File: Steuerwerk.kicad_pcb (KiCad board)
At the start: 2 copper layers, 100 x 160 mm, 332 parts, among them J1 Conn_01x04, J2 Conn_01x02, J3 Conn_01x03, J4 Conn_01x03, J5 Conn_01x02, J6 Conn_01x04, J7 Conn_01x02, J8 Conn_01x04, J9 Conn_01x02, Q1 Q_PNP_BCE, U1 74LS161, U2 74LS138, U3 74LS138, U4 74240, U5 74LS374, U6 74LS374, U7 74541, U8 74541

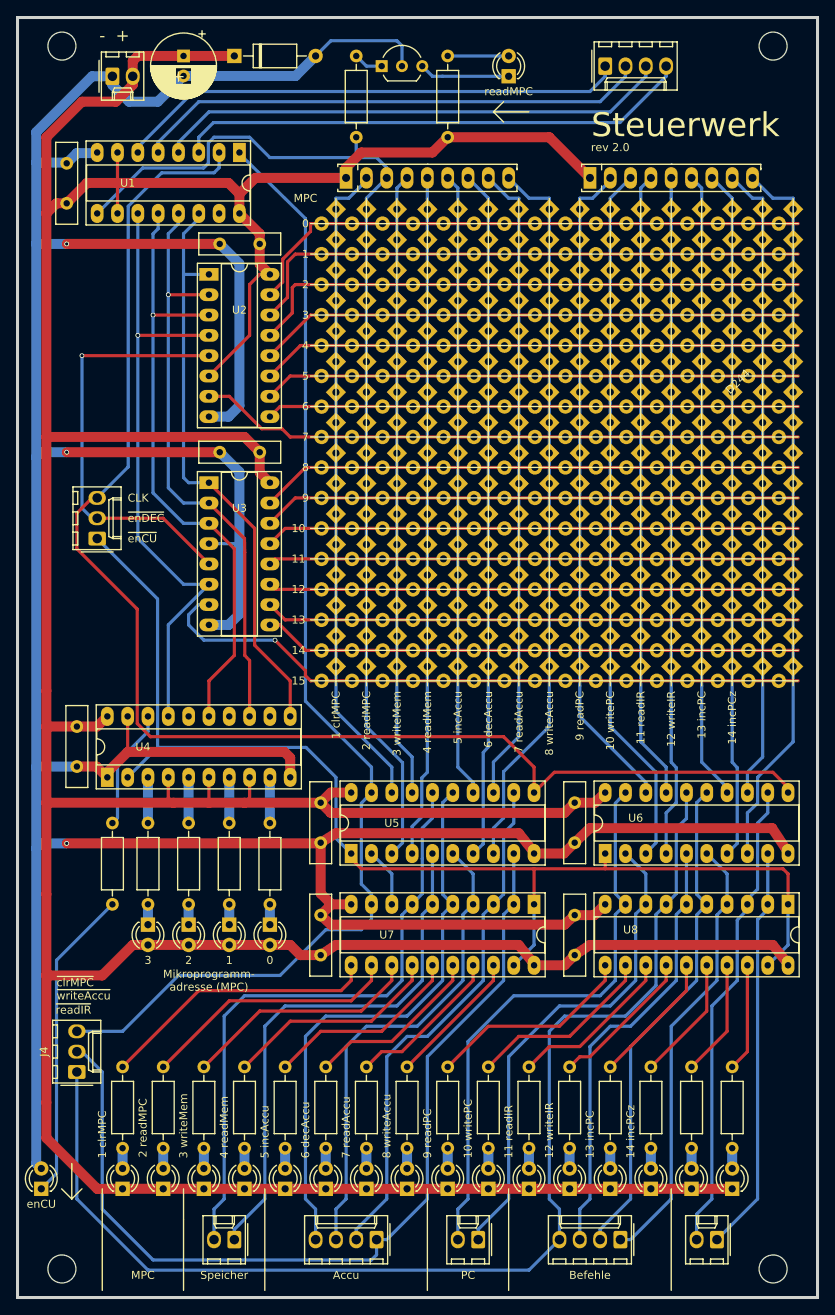
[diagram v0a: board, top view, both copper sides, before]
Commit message: Steuerwerk und Befehle bearbeitet
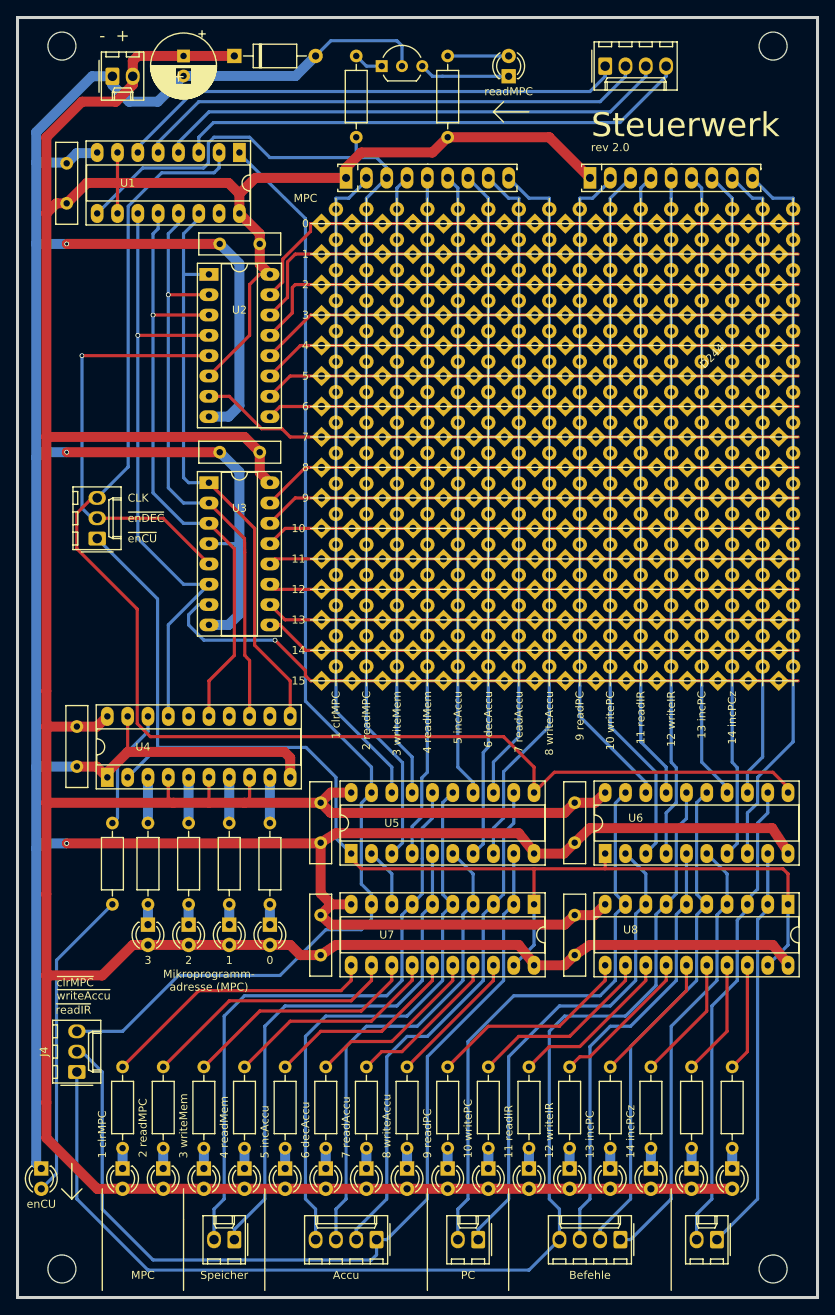
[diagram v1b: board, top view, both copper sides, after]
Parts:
- moved D12 2.55 mm to (87.1, 73.6), turned to 45 degrees
- moved D17 2.55 mm to (125.2, 77.4), turned to 45 degrees
- moved D41 2.55 mm to (121.4, 111.7), turned to 45 degrees
- moved D40 2.54 mm to (87.1, 111.7), turned to 45 degrees
- moved D47 2.54 mm to (44.5, 176.5), turned to 270 degrees
- moved D48 2.54 mm to (54.6, 176.5), turned to 270 degrees
- moved D49 2.54 mm to (59.7, 176.5), turned to 270 degrees
- moved D50 2.54 mm to (64.8, 176.5), turned to 270 degrees
- moved D51 2.54 mm to (69.9, 176.5), turned to 270 degrees
- moved D52 2.54 mm to (75.0, 176.5), turned to 270 degrees
- moved D53 2.54 mm to (80.0, 176.5), turned to 270 degrees
- moved D54 2.54 mm to (85.1, 176.5), turned to 270 degrees
- moved D55 2.54 mm to (90.2, 176.5), turned to 270 degrees
- moved D56 2.54 mm to (95.3, 176.5), turned to 270 degrees
- moved D57 2.54 mm to (100.4, 176.5), turned to 270 degrees
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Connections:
- D10 pad 1: Net-(D10-Pad1) -> /h6
- D10 pad 2: /h6 -> Net-(D10-Pad2)
- D100 pad 1: Net-(D100-Pad1) -> /h5
- D100 pad 2: /h5 -> Net-(D100-Pad2)
- D101 pad 1: Net-(D101-Pad1) -> /h5
- D101 pad 2: /h5 -> Net-(D101-Pad2)
- D102 pad 1: Net-(D102-Pad1) -> /h5
- D102 pad 2: /h5 -> Net-(D102-Pad2)
- D103 pad 1: Net-(D103-Pad1) -> /h5
- D103 pad 2: /h5 -> Net-(D103-Pad2)
- D104 pad 1: Net-(D104-Pad1) -> /h5
- D104 pad 2: /h5 -> Net-(D104-Pad2)
- D105 pad 1: Net-(D105-Pad1) -> /h5
- D105 pad 2: /h5 -> Net-(D105-Pad2)
- D106 pad 1: Net-(D100-Pad1) -> /h6
- D106 pad 2: /h6 -> Net-(D100-Pad2)
- D107 pad 1: Net-(D101-Pad1) -> /h6
- D107 pad 2: /h6 -> Net-(D101-Pad2)
- D108 pad 1: Net-(D108-Pad1) -> /h6
- D108 pad 2: /h6 -> Net-(D108-Pad2)
- D109 pad 1: Net-(D103-Pad1) -> /h6
- D109 pad 2: /h6 -> Net-(D103-Pad2)
- D11 pad 1: Net-(D11-Pad1) -> /h3
- D11 pad 2: /h3 -> Net-(D11-Pad2)
- D110 pad 1: Net-(D104-Pad1) -> /h6
- D110 pad 2: /h6 -> Net-(D104-Pad2)
- D111 pad 1: Net-(D10-Pad1) -> /h7
- D111 pad 2: /h7 -> Net-(D10-Pad2)
- D112 pad 1: Net-(D100-Pad1) -> /h7
- D112 pad 2: /h7 -> Net-(D100-Pad2)
- D113 pad 1: Net-(D101-Pad1) -> /h7
- D113 pad 2: /h7 -> Net-(D101-Pad2)
- D114 pad 1: Net-(D102-Pad1) -> /h7
- D114 pad 2: /h7 -> Net-(D102-Pad2)
- D115 pad 1: Net-(D108-Pad1) -> /h7
- D115 pad 2: /h7 -> Net-(D108-Pad2)
- D116 pad 1: Net-(D103-Pad1) -> /h7
- D116 pad 2: /h7 -> Net-(D103-Pad2)
- D117 pad 1: Net-(D104-Pad1) -> /h7
- D117 pad 2: /h7 -> Net-(D104-Pad2)
- D118 pad 1: Net-(D105-Pad1) -> /h7
- D118 pad 2: /h7 -> Net-(D105-Pad2)
- D119 pad 1: Net-(D10-Pad1) -> /h8
- D119 pad 2: /h8 -> Net-(D10-Pad2)
- D12 pad 1: Net-(D101-Pad1) -> /h4
- D12 pad 2: /h4 -> Net-(D101-Pad2)
- D120 pad 1: Net-(D100-Pad1) -> /h8
- D120 pad 2: /h8 -> Net-(D100-Pad2)
- D121 pad 1: Net-(D102-Pad1) -> /h8
- D121 pad 2: /h8 -> Net-(D102-Pad2)
- D122 pad 1: Net-(D108-Pad1) -> /h8
- D122 pad 2: /h8 -> Net-(D108-Pad2)
- D123 pad 1: Net-(D103-Pad1) -> /h8
- D123 pad 2: /h8 -> Net-(D103-Pad2)
- D124 pad 1: Net-(D105-Pad1) -> /h8
- D124 pad 2: /h8 -> Net-(D105-Pad2)
- D125 pad 1: Net-(D10-Pad1) -> /h9
- D125 pad 2: /h9 -> Net-(D10-Pad2)
- D126 pad 1: Net-(D100-Pad1) -> /h9
- D126 pad 2: /h9 -> Net-(D100-Pad2)
- D127 pad 1: Net-(D101-Pad1) -> /h9
- D127 pad 2: /h9 -> Net-(D101-Pad2)
- D128 pad 1: Net-(D102-Pad1) -> /h9
- D128 pad 2: /h9 -> Net-(D102-Pad2)
- D129 pad 1: Net-(D108-Pad1) -> /h9
- D129 pad 2: /h9 -> Net-(D108-Pad2)
- D13 pad 1: Net-(D104-Pad1) -> /h4
- D13 pad 2: /h4 -> Net-(D104-Pad2)
- D130 pad 1: Net-(D104-Pad1) -> /h9
- D130 pad 2: /h9 -> Net-(D104-Pad2)
- D131 pad 1: Net-(D105-Pad1) -> /h9
- D131 pad 2: /h9 -> Net-(D105-Pad2)
- D132 pad 1: Net-(D100-Pad1) -> /h10
- D132 pad 2: /h10 -> Net-(D100-Pad2)
- D133 pad 1: Net-(D101-Pad1) -> /h10
- D133 pad 2: /h10 -> Net-(D101-Pad2)
- D134 pad 1: Net-(D108-Pad1) -> /h10
- D134 pad 2: /h10 -> Net-(D108-Pad2)
- D135 pad 1: Net-(D103-Pad1) -> /h10
- D135 pad 2: /h10 -> Net-(D103-Pad2)
- D136 pad 1: Net-(D104-Pad1) -> /h10
- D136 pad 2: /h10 -> Net-(D104-Pad2)
- D137 pad 1: Net-(D100-Pad1) -> /h11
- D137 pad 2: /h11 -> Net-(D100-Pad2)
- D138 pad 1: Net-(D101-Pad1) -> /h11
- D138 pad 2: /h11 -> Net-(D101-Pad2)
- D139 pad 1: Net-(D102-Pad1) -> /h11
- D139 pad 2: /h11 -> Net-(D102-Pad2)
- D14 pad 1: Net-(D11-Pad1) -> /h4
- D14 pad 2: /h4 -> Net-(D11-Pad2)
- D140 pad 1: Net-(D108-Pad1) -> /h11
- D140 pad 2: /h11 -> Net-(D108-Pad2)
- D141 pad 1: Net-(D103-Pad1) -> /h11
- D141 pad 2: /h11 -> Net-(D103-Pad2)
- D142 pad 1: Net-(D104-Pad1) -> /h11
- D142 pad 2: /h11 -> Net-(D104-Pad2)
- D143 pad 1: Net-(D105-Pad1) -> /h11
- D143 pad 2: /h11 -> Net-(D105-Pad2)
- D144 pad 1: Net-(D10-Pad1) -> /h12
- D144 pad 2: /h12 -> Net-(D10-Pad2)
- D145 pad 1: Net-(D100-Pad1) -> /h12
- D145 pad 2: /h12 -> Net-(D100-Pad2)
- D146 pad 1: Net-(D101-Pad1) -> /h12
- D146 pad 2: /h12 -> Net-(D101-Pad2)
- D147 pad 1: Net-(D102-Pad1) -> /h12
- D147 pad 2: /h12 -> Net-(D102-Pad2)
- D148 pad 1: Net-(D108-Pad1) -> /h12
- D148 pad 2: /h12 -> Net-(D108-Pad2)
- D149 pad 1: Net-(D103-Pad1) -> /h12
- D149 pad 2: /h12 -> Net-(D103-Pad2)
- D15 pad 1: Net-(D108-Pad1) -> /h5
- D15 pad 2: /h5 -> Net-(D108-Pad2)
- D150 pad 1: Net-(D104-Pad1) -> /h12
- D150 pad 2: /h12 -> Net-(D104-Pad2)
- D151 pad 1: Net-(D105-Pad1) -> /h12
- D151 pad 2: /h12 -> Net-(D105-Pad2)
- D152 pad 1: Net-(D10-Pad1) -> /h13
- D152 pad 2: /h13 -> Net-(D10-Pad2)
- D153 pad 1: Net-(D100-Pad1) -> /h13
- D153 pad 2: /h13 -> Net-(D100-Pad2)
- D154 pad 1: Net-(D102-Pad1) -> /h13
- D154 pad 2: /h13 -> Net-(D102-Pad2)
- D155 pad 1: Net-(D108-Pad1) -> /h13
- D155 pad 2: /h13 -> Net-(D108-Pad2)
- D156 pad 1: Net-(D103-Pad1) -> /h13
- D156 pad 2: /h13 -> Net-(D103-Pad2)
- D157 pad 1: Net-(D104-Pad1) -> /h13
- D157 pad 2: /h13 -> Net-(D104-Pad2)
- D158 pad 1: Net-(D105-Pad1) -> /h13
- D158 pad 2: /h13 -> Net-(D105-Pad2)
- D159 pad 1: Net-(D100-Pad1) -> /h14
- D159 pad 2: /h14 -> Net-(D100-Pad2)
- D16 pad 1: Net-(D11-Pad1) -> /h5
- D16 pad 2: /h5 -> Net-(D11-Pad2)
- D160 pad 1: Net-(D102-Pad1) -> /h14
- D160 pad 2: /h14 -> Net-(D102-Pad2)
- D161 pad 1: Net-(D108-Pad1) -> /h14
- D161 pad 2: /h14 -> Net-(D108-Pad2)
- D162 pad 1: Net-(D103-Pad1) -> /h14
- D162 pad 2: /h14 -> Net-(D103-Pad2)
- D163 pad 1: Net-(D104-Pad1) -> /h14
- D163 pad 2: /h14 -> Net-(D104-Pad2)
- D164 pad 1: Net-(D105-Pad1) -> /h14
- D164 pad 2: /h14 -> Net-(D105-Pad2)
- D165 pad 1: Net-(D10-Pad1) -> /h15
- D165 pad 2: /h15 -> Net-(D10-Pad2)
- D166 pad 1: Net-(D100-Pad1) -> /h15
- D166 pad 2: /h15 -> Net-(D100-Pad2)
- D167 pad 1: Net-(D101-Pad1) -> /h15
- D167 pad 2: /h15 -> Net-(D101-Pad2)
- D168 pad 1: Net-(D102-Pad1) -> /h15
- D168 pad 2: /h15 -> Net-(D102-Pad2)
- D169 pad 1: Net-(D108-Pad1) -> /h15
- D169 pad 2: /h15 -> Net-(D108-Pad2)
- D17 pad 1: Net-(D17-Pad1) -> /h5
- D17 pad 2: /h5 -> Net-(D17-Pad2)
- D170 pad 1: Net-(D103-Pad1) -> /h15
- D170 pad 2: /h15 -> Net-(D103-Pad2)
- D171 pad 1: Net-(D104-Pad1) -> /h15
- D171 pad 2: /h15 -> Net-(D104-Pad2)
- D172 pad 1: Net-(D105-Pad1) -> /h15
- D172 pad 2: /h15 -> Net-(D105-Pad2)
- D173 pad 1: Net-(D173-Pad1) -> /h0
- D173 pad 2: /h0 -> Net-(D173-Pad2)
- D174 pad 1: Net-(D174-Pad1) -> /h0
- D174 pad 2: /h0 -> Net-(D174-Pad2)
- D175 pad 1: Net-(D11-Pad1) -> /h0
- D175 pad 2: /h0 -> Net-(D11-Pad2)
- D176 pad 1: Net-(D17-Pad1) -> /h0
- D176 pad 2: /h0 -> Net-(D17-Pad2)
- D177 pad 1: Net-(D177-Pad1) -> /h0
- D177 pad 2: /h0 -> Net-(D177-Pad2)
- D178 pad 1: Net-(D178-Pad1) -> /h0
- D178 pad 2: /h0 -> Net-(D178-Pad2)
- D179 pad 1: Net-(D179-Pad1) -> /h0
- D179 pad 2: /h0 -> Net-(D179-Pad2)
- D18 pad 1: Net-(D102-Pad1) -> /h6
- D18 pad 2: /h6 -> Net-(D102-Pad2)
- D180 pad 1: Net-(D173-Pad1) -> /h1
- D180 pad 2: /h1 -> Net-(D173-Pad2)
- D181 pad 1: Net-(D11-Pad1) -> /h1
- D181 pad 2: /h1 -> Net-(D11-Pad2)
- D182 pad 1: Net-(D17-Pad1) -> /h1
- D182 pad 2: /h1 -> Net-(D17-Pad2)
- D183 pad 1: Net-(D177-Pad1) -> /h1
- D183 pad 2: /h1 -> Net-(D177-Pad2)
- D184 pad 1: Net-(D178-Pad1) -> /h1
- D184 pad 2: /h1 -> Net-(D178-Pad2)
- D185 pad 1: Net-(D179-Pad1) -> /h1
- D185 pad 2: /h1 -> Net-(D179-Pad2)
- D186 pad 1: Net-(D173-Pad1) -> /h2
- D186 pad 2: /h2 -> Net-(D173-Pad2)
- D187 pad 1: Net-(D174-Pad1) -> /h2
- D187 pad 2: /h2 -> Net-(D174-Pad2)
- D188 pad 1: Net-(D11-Pad1) -> /h2
- D188 pad 2: /h2 -> Net-(D11-Pad2)
- D189 pad 1: Net-(D17-Pad1) -> /h2
- D189 pad 2: /h2 -> Net-(D17-Pad2)
- D19 pad 1: Net-(D105-Pad1) -> /h6
- D19 pad 2: /h6 -> Net-(D105-Pad2)
- D190 pad 1: Net-(D177-Pad1) -> /h2
- D190 pad 2: /h2 -> Net-(D177-Pad2)
- D191 pad 1: Net-(D178-Pad1) -> /h2
- D191 pad 2: /h2 -> Net-(D178-Pad2)
- D192 pad 1: Net-(D179-Pad1) -> /h2
- D192 pad 2: /h2 -> Net-(D179-Pad2)
- D193 pad 1: Net-(D173-Pad1) -> /h3
- D193 pad 2: /h3 -> Net-(D173-Pad2)
- D194 pad 1: Net-(D173-Pad1) -> /h4
- D194 pad 2: /h4 -> Net-(D173-Pad2)
- D195 pad 1: Net-(D173-Pad1) -> /h5
- D195 pad 2: /h5 -> Net-(D173-Pad2)
- D196 pad 1: Net-(D173-Pad1) -> /h6
- D196 pad 2: /h6 -> Net-(D173-Pad2)
- D197 pad 1: Net-(D173-Pad1) -> /h7
- D197 pad 2: /h7 -> Net-(D173-Pad2)
- D198 pad 1: Net-(D173-Pad1) -> /h8
- D198 pad 2: /h8 -> Net-(D173-Pad2)
- D199 pad 1: Net-(D173-Pad1) -> /h9
- D199 pad 2: /h9 -> Net-(D173-Pad2)
- D20 pad 1: Net-(D11-Pad1) -> /h6
- D20 pad 2: /h6 -> Net-(D11-Pad2)
- D200 pad 1: Net-(D173-Pad1) -> /h10
- D200 pad 2: /h10 -> Net-(D173-Pad2)
- D201 pad 1: Net-(D173-Pad1) -> /h12
- D201 pad 2: /h12 -> Net-(D173-Pad2)
- D202 pad 1: Net-(D173-Pad1) -> /h13
- D202 pad 2: /h13 -> Net-(D173-Pad2)
- D203 pad 1: Net-(D173-Pad1) -> /h14
- D203 pad 2: /h14 -> Net-(D173-Pad2)
- D204 pad 1: Net-(D173-Pad1) -> /h15
- D204 pad 2: /h15 -> Net-(D173-Pad2)
- D205 pad 1: Net-(D205-Pad1) -> /h3
- D205 pad 2: /h3 -> Net-(D205-Pad2)
- D206 pad 1: Net-(D205-Pad1) -> /h4
- D206 pad 2: /h4 -> Net-(D205-Pad2)
- D207 pad 1: Net-(D205-Pad1) -> /h5
- D207 pad 2: /h5 -> Net-(D205-Pad2)
- D208 pad 1: Net-(D205-Pad1) -> /h6
- D208 pad 2: /h6 -> Net-(D205-Pad2)
- D209 pad 1: Net-(D205-Pad1) -> /h7
- D209 pad 2: /h7 -> Net-(D205-Pad2)
- D21 pad 1: Net-(D11-Pad1) -> /h7
- D21 pad 2: /h7 -> Net-(D11-Pad2)
- D210 pad 1: Net-(D205-Pad1) -> /h8
- D210 pad 2: /h8 -> Net-(D205-Pad2)
- D211 pad 1: Net-(D205-Pad1) -> /h9
- D211 pad 2: /h9 -> Net-(D205-Pad2)
- D212 pad 1: Net-(D205-Pad1) -> /h10
- D212 pad 2: /h10 -> Net-(D205-Pad2)
- D213 pad 1: Net-(D205-Pad1) -> /h11
- D213 pad 2: /h11 -> Net-(D205-Pad2)
- D214 pad 1: Net-(D205-Pad1) -> /h12
- D214 pad 2: /h12 -> Net-(D205-Pad2)
- D215 pad 1: Net-(D205-Pad1) -> /h13
- D215 pad 2: /h13 -> Net-(D205-Pad2)
- D216 pad 1: Net-(D205-Pad1) -> /h14
- D216 pad 2: /h14 -> Net-(D205-Pad2)
- D217 pad 1: Net-(D205-Pad1) -> /h15
- D217 pad 2: /h15 -> Net-(D205-Pad2)
- D218 pad 1: Net-(D174-Pad1) -> /h3
- D218 pad 2: /h3 -> Net-(D174-Pad2)
- D219 pad 1: Net-(D174-Pad1) -> /h4
- D219 pad 2: /h4 -> Net-(D174-Pad2)
- D22 pad 1: Net-(D101-Pad1) -> /h8
- D22 pad 2: /h8 -> Net-(D101-Pad2)
- D220 pad 1: Net-(D174-Pad1) -> /h5
- D220 pad 2: /h5 -> Net-(D174-Pad2)
- D221 pad 1: Net-(D174-Pad1) -> /h6
- D221 pad 2: /h6 -> Net-(D174-Pad2)
- D222 pad 1: Net-(D174-Pad1) -> /h7
- D222 pad 2: /h7 -> Net-(D174-Pad2)
- D223 pad 1: Net-(D174-Pad1) -> /h8
- D223 pad 2: /h8 -> Net-(D174-Pad2)
- D224 pad 1: Net-(D174-Pad1) -> /h9
- D224 pad 2: /h9 -> Net-(D174-Pad2)
- D225 pad 1: Net-(D174-Pad1) -> /h10
- D225 pad 2: /h10 -> Net-(D174-Pad2)
- D226 pad 1: Net-(D174-Pad1) -> /h11
- D226 pad 2: /h11 -> Net-(D174-Pad2)
- D227 pad 1: Net-(D174-Pad1) -> /h12
- D227 pad 2: /h12 -> Net-(D174-Pad2)
- D228 pad 1: Net-(D174-Pad1) -> /h13
- D228 pad 2: /h13 -> Net-(D174-Pad2)
- D229 pad 1: Net-(D174-Pad1) -> /h14
- D229 pad 2: /h14 -> Net-(D174-Pad2)
- D23 pad 1: Net-(D104-Pad1) -> /h8
- D23 pad 2: /h8 -> Net-(D104-Pad2)
- D230 pad 1: Net-(D174-Pad1) -> /h15
- D230 pad 2: /h15 -> Net-(D174-Pad2)
- D231 pad 1: Net-(D11-Pad1) -> /h15
- D231 pad 2: /h15 -> Net-(D11-Pad2)
- D232 pad 1: Net-(D17-Pad1) -> /h3
- D232 pad 2: /h3 -> Net-(D17-Pad2)
- D233 pad 1: Net-(D17-Pad1) -> /h4
- D233 pad 2: /h4 -> Net-(D17-Pad2)
- D234 pad 1: Net-(D17-Pad1) -> /h6
- D234 pad 2: /h6 -> Net-(D17-Pad2)
- D235 pad 1: Net-(D17-Pad1) -> /h7
- D235 pad 2: /h7 -> Net-(D17-Pad2)
- D236 pad 1: Net-(D17-Pad1) -> /h8
- D236 pad 2: /h8 -> Net-(D17-Pad2)
- D237 pad 1: Net-(D17-Pad1) -> /h10
- D237 pad 2: /h10 -> Net-(D17-Pad2)
- D238 pad 1: Net-(D17-Pad1) -> /h11
- D238 pad 2: /h11 -> Net-(D17-Pad2)
- D239 pad 1: Net-(D17-Pad1) -> /h13
- D239 pad 2: /h13 -> Net-(D17-Pad2)
- D24 pad 1: Net-(D11-Pad1) -> /h8
- D24 pad 2: /h8 -> Net-(D11-Pad2)
- D240 pad 1: Net-(D17-Pad1) -> /h14
- D240 pad 2: /h14 -> Net-(D17-Pad2)
- D241 pad 1: Net-(D17-Pad1) -> /h15
- D241 pad 2: /h15 -> Net-(D17-Pad2)
- D242 pad 1: Net-(D177-Pad1) -> /h3
- D242 pad 2: /h3 -> Net-(D177-Pad2)
- D243 pad 1: Net-(D177-Pad1) -> /h4
- D243 pad 2: /h4 -> Net-(D177-Pad2)
- D244 pad 1: Net-(D177-Pad1) -> /h5
- D244 pad 2: /h5 -> Net-(D177-Pad2)
- D245 pad 1: Net-(D177-Pad1) -> /h6
- D245 pad 2: /h6 -> Net-(D177-Pad2)
- D246 pad 1: Net-(D177-Pad1) -> /h7
- D246 pad 2: /h7 -> Net-(D177-Pad2)
- D247 pad 1: Net-(D177-Pad1) -> /h8
- D247 pad 2: /h8 -> Net-(D177-Pad2)
- D248 pad 1: Net-(D177-Pad1) -> /h9
- D248 pad 2: /h9 -> Net-(D177-Pad2)
- D249 pad 1: Net-(D177-Pad1) -> /h10
- D249 pad 2: /h10 -> Net-(D177-Pad2)
- D25 pad 1: Net-(D103-Pad1) -> /h9
- D25 pad 2: /h9 -> Net-(D103-Pad2)
- D250 pad 1: Net-(D177-Pad1) -> /h11
- D250 pad 2: /h11 -> Net-(D177-Pad2)
- D251 pad 1: Net-(D177-Pad1) -> /h12
- D251 pad 2: /h12 -> Net-(D177-Pad2)
- D252 pad 1: Net-(D177-Pad1) -> /h13
- D252 pad 2: /h13 -> Net-(D177-Pad2)
- D253 pad 1: Net-(D177-Pad1) -> /h15
- D253 pad 2: /h15 -> Net-(D177-Pad2)
- D254 pad 1: Net-(D178-Pad1) -> /h3
- D254 pad 2: /h3 -> Net-(D178-Pad2)
- D255 pad 1: Net-(D179-Pad1) -> /h3
- D255 pad 2: /h3 -> Net-(D179-Pad2)
- D256 pad 1: Net-(D178-Pad1) -> /h4
- D256 pad 2: /h4 -> Net-(D178-Pad2)
- D257 pad 1: Net-(D179-Pad1) -> /h4
- D257 pad 2: /h4 -> Net-(D179-Pad2)
- D258 pad 1: Net-(D178-Pad1) -> /h5
- D258 pad 2: /h5 -> Net-(D178-Pad2)
- D259 pad 1: Net-(D179-Pad1) -> /h5
- D259 pad 2: /h5 -> Net-(D179-Pad2)
- D26 pad 1: Net-(D11-Pad1) -> /h9
- D26 pad 2: /h9 -> Net-(D11-Pad2)
- D260 pad 1: Net-(D178-Pad1) -> /h6
- D260 pad 2: /h6 -> Net-(D178-Pad2)
- D261 pad 1: Net-(D179-Pad1) -> /h6
- D261 pad 2: /h6 -> Net-(D179-Pad2)
- D262 pad 1: Net-(D178-Pad1) -> /h7
- D262 pad 2: /h7 -> Net-(D178-Pad2)
- D263 pad 1: Net-(D179-Pad1) -> /h7
- D263 pad 2: /h7 -> Net-(D179-Pad2)
- D264 pad 1: Net-(D178-Pad1) -> /h8
- D264 pad 2: /h8 -> Net-(D178-Pad2)
- D265 pad 1: Net-(D179-Pad1) -> /h8
- D265 pad 2: /h8 -> Net-(D179-Pad2)
- D266 pad 1: Net-(D178-Pad1) -> /h9
- D266 pad 2: /h9 -> Net-(D178-Pad2)
- D267 pad 1: Net-(D179-Pad1) -> /h9
- D267 pad 2: /h9 -> Net-(D179-Pad2)
- D268 pad 1: Net-(D178-Pad1) -> /h10
- D268 pad 2: /h10 -> Net-(D178-Pad2)
- D269 pad 1: Net-(D179-Pad1) -> /h10
- D269 pad 2: /h10 -> Net-(D179-Pad2)
- D27 pad 1: Net-(D17-Pad1) -> /h9
- D27 pad 2: /h9 -> Net-(D17-Pad2)
- D270 pad 1: Net-(D178-Pad1) -> /h11
- D270 pad 2: /h11 -> Net-(D178-Pad2)
- D271 pad 1: Net-(D179-Pad1) -> /h11
- D271 pad 2: /h11 -> Net-(D179-Pad2)
- D272 pad 1: Net-(D178-Pad1) -> /h12
- D272 pad 2: /h12 -> Net-(D178-Pad2)
- D273 pad 1: Net-(D179-Pad1) -> /h12
- D273 pad 2: /h12 -> Net-(D179-Pad2)
- D274 pad 1: Net-(D178-Pad1) -> /h13
- D274 pad 2: /h13 -> Net-(D178-Pad2)
- D275 pad 1: Net-(D179-Pad1) -> /h13
- D275 pad 2: /h13 -> Net-(D179-Pad2)
- D276 pad 1: Net-(D178-Pad1) -> /h14
- D276 pad 2: /h14 -> Net-(D178-Pad2)
- D277 pad 1: Net-(D179-Pad1) -> /h14
- D277 pad 2: /h14 -> Net-(D179-Pad2)
- D278 pad 1: Net-(D178-Pad1) -> /h15
- D278 pad 2: /h15 -> Net-(D178-Pad2)
- D279 pad 1: Net-(D179-Pad1) -> /h15
- D279 pad 2: /h15 -> Net-(D179-Pad2)
- D28 pad 1: Net-(D10-Pad1) -> /h10
- D28 pad 2: /h10 -> Net-(D10-Pad2)
- D29 pad 1: Net-(D102-Pad1) -> /h10
- D29 pad 2: /h10 -> Net-(D102-Pad2)
- D3 pad 1: Net-(D101-Pad1) -> /h1
- D3 pad 2: /h1 -> Net-(D101-Pad2)
- D30 pad 1: Net-(D105-Pad1) -> /h10
- D30 pad 2: /h10 -> Net-(D105-Pad2)
- D31 pad 1: Net-(D11-Pad1) -> /h10
- D31 pad 2: /h10 -> Net-(D11-Pad2)
- D32 pad 1: Net-(D10-Pad1) -> /h11
- D32 pad 2: /h11 -> Net-(D10-Pad2)
- D33 pad 1: Net-(D173-Pad1) -> /h11
- D33 pad 2: /h11 -> Net-(D173-Pad2)
- D34 pad 1: Net-(D11-Pad1) -> /h11
- D34 pad 2: /h11 -> Net-(D11-Pad2)
- D35 pad 1: Net-(D11-Pad1) -> /h12
- D35 pad 2: /h12 -> Net-(D11-Pad2)
- D36 pad 1: Net-(D17-Pad1) -> /h12
- D36 pad 2: /h12 -> Net-(D17-Pad2)
- D37 pad 1: Net-(D101-Pad1) -> /h13
- D37 pad 2: /h13 -> Net-(D101-Pad2)
- D38 pad 1: Net-(D11-Pad1) -> /h13
- D38 pad 2: /h13 -> Net-(D11-Pad2)
- D39 pad 1: Net-(D10-Pad1) -> /h14
- D39 pad 2: /h14 -> Net-(D10-Pad2)
- D4 pad 1: Net-(D205-Pad1) -> /h0
- D4 pad 2: /h0 -> Net-(D205-Pad2)
- D40 pad 1: Net-(D101-Pad1) -> /h14
- D40 pad 2: /h14 -> Net-(D101-Pad2)
- D41 pad 1: Net-(D11-Pad1) -> /h14
- D41 pad 2: /h14 -> Net-(D11-Pad2)
- D42 pad 1: Net-(D177-Pad1) -> /h14
- D42 pad 2: /h14 -> Net-(D177-Pad2)
- D47 pad 1: Net-(D47-Pad1) -> GND
- D47 pad 2: GND -> Net-(D47-Pad2)
- D48 pad 1: VCC -> Net-(D48-Pad1)
- D48 pad 2: Net-(D48-Pad2) -> VCC
- D49 pad 1: VCC -> Net-(D49-Pad1)
- D49 pad 2: Net-(D49-Pad2) -> VCC
- D5 pad 1: Net-(D205-Pad1) -> /h1
- D5 pad 2: /h1 -> Net-(D205-Pad2)
- D50 pad 1: VCC -> Net-(D50-Pad1)
- D50 pad 2: Net-(D50-Pad2) -> VCC
- D51 pad 1: VCC -> Net-(D51-Pad1)
- D51 pad 2: Net-(D51-Pad2) -> VCC
- D52 pad 1: VCC -> Net-(D52-Pad1)
- D52 pad 2: Net-(D52-Pad2) -> VCC
- D53 pad 1: VCC -> Net-(D53-Pad1)
- D53 pad 2: Net-(D53-Pad2) -> VCC
- D54 pad 1: VCC -> Net-(D54-Pad1)
- D54 pad 2: Net-(D54-Pad2) -> VCC
- D55 pad 1: VCC -> Net-(D55-Pad1)
- D55 pad 2: Net-(D55-Pad2) -> VCC
- D56 pad 1: VCC -> Net-(D56-Pad1)
- D56 pad 2: Net-(D56-Pad2) -> VCC
- D57 pad 1: VCC -> Net-(D57-Pad1)
- D57 pad 2: Net-(D57-Pad2) -> VCC
- D58 pad 1: VCC -> Net-(D58-Pad1)
- D58 pad 2: Net-(D58-Pad2) -> VCC
- D59 pad 1: VCC -> Net-(D59-Pad1)
- D59 pad 2: Net-(D59-Pad2) -> VCC
- D6 pad 1: Net-(D174-Pad1) -> /h1
- D6 pad 2: /h1 -> Net-(D174-Pad2)
- D60 pad 1: VCC -> Net-(D60-Pad1)
- D60 pad 2: Net-(D60-Pad2) -> VCC
- D61 pad 1: VCC -> Net-(D61-Pad1)
- D61 pad 2: Net-(D61-Pad2) -> VCC
- D62 pad 1: VCC -> Net-(D62-Pad1)
- D62 pad 2: Net-(D62-Pad2) -> VCC
- D63 pad 1: VCC -> Net-(D63-Pad1)
- D63 pad 2: Net-(D63-Pad2) -> VCC
- D64 pad 1: Net-(D10-Pad1) -> /h0
- D64 pad 2: /h0 -> Net-(D10-Pad2)
- D65 pad 1: Net-(D100-Pad1) -> /h0
- D65 pad 2: /h0 -> Net-(D100-Pad2)
- D66 pad 1: Net-(D101-Pad1) -> /h0
- D66 pad 2: /h0 -> Net-(D101-Pad2)
- D67 pad 1: Net-(D102-Pad1) -> /h0
- D67 pad 2: /h0 -> Net-(D102-Pad2)
- D68 pad 1: Net-(D108-Pad1) -> /h0
- D68 pad 2: /h0 -> Net-(D108-Pad2)
- D69 pad 1: Net-(D103-Pad1) -> /h0
- D69 pad 2: /h0 -> Net-(D103-Pad2)
- D7 pad 1: Net-(D100-Pad1) -> /h2
- D7 pad 2: /h2 -> Net-(D100-Pad2)
- D70 pad 1: Net-(D104-Pad1) -> /h0
- D70 pad 2: /h0 -> Net-(D104-Pad2)
- D71 pad 1: Net-(D105-Pad1) -> /h0
- D71 pad 2: /h0 -> Net-(D105-Pad2)
- D72 pad 1: Net-(D10-Pad1) -> /h1
- D72 pad 2: /h1 -> Net-(D10-Pad2)
- D73 pad 1: Net-(D100-Pad1) -> /h1
- D73 pad 2: /h1 -> Net-(D100-Pad2)
- D74 pad 1: Net-(D102-Pad1) -> /h1
- D74 pad 2: /h1 -> Net-(D102-Pad2)
- D75 pad 1: Net-(D108-Pad1) -> /h1
- D75 pad 2: /h1 -> Net-(D108-Pad2)
- D76 pad 1: Net-(D103-Pad1) -> /h1
- D76 pad 2: /h1 -> Net-(D103-Pad2)
- D77 pad 1: Net-(D104-Pad1) -> /h1
- D77 pad 2: /h1 -> Net-(D104-Pad2)
- D78 pad 1: Net-(D105-Pad1) -> /h1
- D78 pad 2: /h1 -> Net-(D105-Pad2)
- D79 pad 1: Net-(D10-Pad1) -> /h2
- D79 pad 2: /h2 -> Net-(D10-Pad2)
- D8 pad 1: Net-(D101-Pad1) -> /h2
- D8 pad 2: /h2 -> Net-(D101-Pad2)
- D80 pad 1: Net-(D102-Pad1) -> /h2
- D80 pad 2: /h2 -> Net-(D102-Pad2)
- D81 pad 1: Net-(D108-Pad1) -> /h2
- D81 pad 2: /h2 -> Net-(D108-Pad2)
- D82 pad 1: Net-(D103-Pad1) -> /h2
- D82 pad 2: /h2 -> Net-(D103-Pad2)
- D83 pad 1: Net-(D104-Pad1) -> /h2
- D83 pad 2: /h2 -> Net-(D104-Pad2)
- D84 pad 1: Net-(D105-Pad1) -> /h2
- D84 pad 2: /h2 -> Net-(D105-Pad2)
- D85 pad 1: Net-(D10-Pad1) -> /h3
- D85 pad 2: /h3 -> Net-(D10-Pad2)
- D86 pad 1: Net-(D100-Pad1) -> /h3
- D86 pad 2: /h3 -> Net-(D100-Pad2)
- D87 pad 1: Net-(D101-Pad1) -> /h3
- D87 pad 2: /h3 -> Net-(D101-Pad2)
- D88 pad 1: Net-(D102-Pad1) -> /h3
- D88 pad 2: /h3 -> Net-(D102-Pad2)
- D89 pad 1: Net-(D108-Pad1) -> /h3
- D89 pad 2: /h3 -> Net-(D108-Pad2)
- D9 pad 1: Net-(D205-Pad1) -> /h2
- D9 pad 2: /h2 -> Net-(D205-Pad2)
- D90 pad 1: Net-(D103-Pad1) -> /h3
- D90 pad 2: /h3 -> Net-(D103-Pad2)
- D91 pad 1: Net-(D104-Pad1) -> /h3
- D91 pad 2: /h3 -> Net-(D104-Pad2)
- D92 pad 1: Net-(D105-Pad1) -> /h3
- D92 pad 2: /h3 -> Net-(D105-Pad2)
- D93 pad 1: Net-(D10-Pad1) -> /h4
- D93 pad 2: /h4 -> Net-(D10-Pad2)
- D94 pad 1: Net-(D100-Pad1) -> /h4
- D94 pad 2: /h4 -> Net-(D100-Pad2)
- D95 pad 1: Net-(D102-Pad1) -> /h4
- D95 pad 2: /h4 -> Net-(D102-Pad2)
- D96 pad 1: Net-(D108-Pad1) -> /h4
- D96 pad 2: /h4 -> Net-(D108-Pad2)
- D97 pad 1: Net-(D103-Pad1) -> /h4
- D97 pad 2: /h4 -> Net-(D103-Pad2)
- D98 pad 1: Net-(D105-Pad1) -> /h4
- D98 pad 2: /h4 -> Net-(D105-Pad2)
- D99 pad 1: Net-(D10-Pad1) -> /h5
- D99 pad 2: /h5 -> Net-(D10-Pad2)
- R10 pad 2: Net-(D50-Pad2) -> Net-(D50-Pad1)
- R11 pad 2: Net-(D51-Pad2) -> Net-(D51-Pad1)
- R12 pad 2: Net-(D52-Pad2) -> Net-(D52-Pad1)
- R13 pad 2: Net-(D53-Pad2) -> Net-(D53-Pad1)
- R14 pad 2: Net-(D54-Pad2) -> Net-(D54-Pad1)
- R15 pad 2: Net-(D55-Pad2) -> Net-(D55-Pad1)
- R16 pad 2: Net-(D56-Pad2) -> Net-(D56-Pad1)
- R17 pad 2: Net-(D57-Pad2) -> Net-(D57-Pad1)
- R18 pad 2: Net-(D58-Pad2) -> Net-(D58-Pad1)
- R19 pad 2: Net-(D59-Pad2) -> Net-(D59-Pad1)
- R2 pad 2: Net-(D100-Pad1) -> Net-(D100-Pad2)
- R20 pad 2: Net-(D60-Pad2) -> Net-(D60-Pad1)
- R21 pad 2: Net-(D61-Pad2) -> Net-(D61-Pad1)
- R22 pad 2: Net-(D62-Pad2) -> Net-(D62-Pad1)
- R23 pad 2: Net-(D63-Pad2) -> Net-(D63-Pad1)
- R7 pad 2: Net-(D47-Pad1) -> Net-(D47-Pad2)
- R8 pad 2: Net-(D48-Pad2) -> Net-(D48-Pad1)
- R9 pad 2: Net-(D49-Pad2) -> Net-(D49-Pad1)
- RP1 pad 2: Net-(D10-Pad1) -> Net-(D10-Pad2)
- RP1 pad 3: Net-(D100-Pad1) -> Net-(D100-Pad2)
- RP1 pad 4: Net-(D101-Pad1) -> Net-(D101-Pad2)
- RP1 pad 5: Net-(D102-Pad1) -> Net-(D102-Pad2)
- RP1 pad 6: Net-(D108-Pad1) -> Net-(D108-Pad2)
- RP1 pad 7: Net-(D103-Pad1) -> Net-(D103-Pad2)
- RP1 pad 8: Net-(D104-Pad1) -> Net-(D104-Pad2)
- RP1 pad 9: Net-(D105-Pad1) -> Net-(D105-Pad2)
- RP2 pad 2: Net-(D173-Pad1) -> Net-(D173-Pad2)
- RP2 pad 3: Net-(D205-Pad1) -> Net-(D205-Pad2)
- RP2 pad 4: Net-(D174-Pad1) -> Net-(D174-Pad2)
- RP2 pad 5: Net-(D11-Pad1) -> Net-(D11-Pad2)
- RP2 pad 6: Net-(D17-Pad1) -> Net-(D17-Pad2)
- RP2 pad 7: Net-(D177-Pad1) -> Net-(D177-Pad2)
- RP2 pad 8: Net-(D178-Pad1) -> Net-(D178-Pad2)
- RP2 pad 9: Net-(D179-Pad1) -> Net-(D179-Pad2)
- U1 pad 9: Net-(D100-Pad1) -> Net-(D100-Pad2)
- U5 pad 13: Net-(D104-Pad1) -> Net-(D104-Pad2)
- U5 pad 14: Net-(D108-Pad1) -> Net-(D108-Pad2)
- U5 pad 17: Net-(D101-Pad1) -> Net-(D101-Pad2)
- U5 pad 18: Net-(D10-Pad1) -> Net-(D10-Pad2)
- U5 pad 3: Net-(D100-Pad1) -> Net-(D100-Pad2)
- U5 pad 4: Net-(D102-Pad1) -> Net-(D102-Pad2)
- U5 pad 7: Net-(D103-Pad1) -> Net-(D103-Pad2)
- U5 pad 8: Net-(D105-Pad1) -> Net-(D105-Pad2)
- U6 pad 13: Net-(D178-Pad1) -> Net-(D178-Pad2)
- U6 pad 14: Net-(D17-Pad1) -> Net-(D17-Pad2)
- U6 pad 17: Net-(D174-Pad1) -> Net-(D174-Pad2)
- U6 pad 18: Net-(D173-Pad1) -> Net-(D173-Pad2)
- U6 pad 3: Net-(D205-Pad1) -> Net-(D205-Pad2)
- U6 pad 4: Net-(D11-Pad1) -> Net-(D11-Pad2)
- U6 pad 7: Net-(D177-Pad1) -> Net-(D177-Pad2)
- U6 pad 8: Net-(D179-Pad1) -> Net-(D179-Pad2)
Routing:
- net Net-(D100-Pad2): track 0.00 -> 134.9 mm
- net Net-(D100-Pad1): track 134.9 -> 0.00 mm
- net Net-(D105-Pad2): track 0.00 -> 91.0 mm
- net Net-(D105-Pad1): track 91.0 -> 0.00 mm
- net Net-(D179-Pad2): track 0.00 -> 90.4 mm
- net Net-(D179-Pad1): track 90.4 -> 0.00 mm
- net Net-(D205-Pad2): track 0.00 -> 88.4 mm
- net Net-(D205-Pad1): track 88.4 -> 0.00 mm
- net Net-(D103-Pad2): track 0.00 -> 86.3 mm
- net Net-(D103-Pad1): track 86.3 -> 0.00 mm
- net Net-(D177-Pad2): track 0.00 -> 86.3 mm
- net Net-(D177-Pad1): track 86.3 -> 0.00 mm
- net Net-(D102-Pad2): track 0.00 -> 85.2 mm
- net Net-(D102-Pad1): track 85.2 -> 0.00 mm
- net Net-(D11-Pad2): track 0.00 -> 85.2 mm
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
